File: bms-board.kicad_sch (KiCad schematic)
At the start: 1 part, among them U1 LTC6804-2

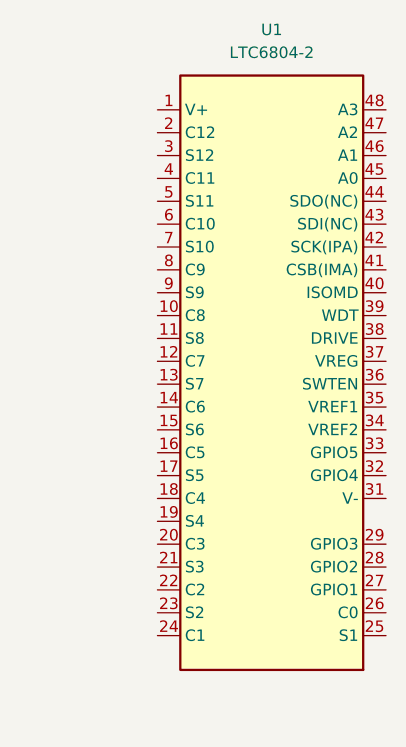
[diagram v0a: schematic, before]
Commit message: Release/0.1 (#8)
* feat: add 6804-2 kicad symbol

* feat: add 6804-2 kicad symbol (#3)

* TEMPLATE: add pull request description template

* feat: add automated git flow setup script

* update feature/add-cells branch to latest develop edition (#4)

* feat: add 6804-2 kicad symbol

* TEMPLATE: add pull request description template

* feat: add automated git flow setup script

* update feature/our-symbol-library branch to latest develop edition (#5)

* TEMPLATE: add pull request description template

* feat: add automated git flow setup script

* feat: a maybe working fixed wing schematic symbol library

* feat: add line to checkout dev branch when running setup script

* feat: fix FixedWing symbol library to include LTC6804-2

* refactor: verifying symbol library works, remove individual ltc6804-2 symbol

* feat: adding needed files

* feat: edit conflict in setup script

* Merging new develop into new feature (#6)

* feat: add 6804-2 kicad symbol

* TEMPLATE: add pull request description template

* feat: add automated git flow setup script

* update feature/our-symbol-library branch to latest develop edition (#5)

* TEMPLATE: add pull request description template

* feat: add automated git flow setup script

* feat: a maybe working fixed wing schematic symbol library

* feat: add line to checkout dev branch when running setup script

* feat: fix FixedWing symbol library to include LTC6804-2

* refactor: verifying symbol library works, remove individual ltc6804-2 symbol

* feat: adding needed files

* feat: edit conflict in setup script

---------

Co-authored-by: Ephram Cola Jacquin <89238547+ephram2004@users.noreply.github.com>
Co-authored-by: Ephram Cola Jacquin <ecolajacquin@gmail.com>

* fix: changed symbol for easier schematic design and orginization by pin logic

* docs: Update pull_request_template.md

---------

Co-authored-by: Ephram Cola Jacquin <89238547+ephram2004@users.noreply.gith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
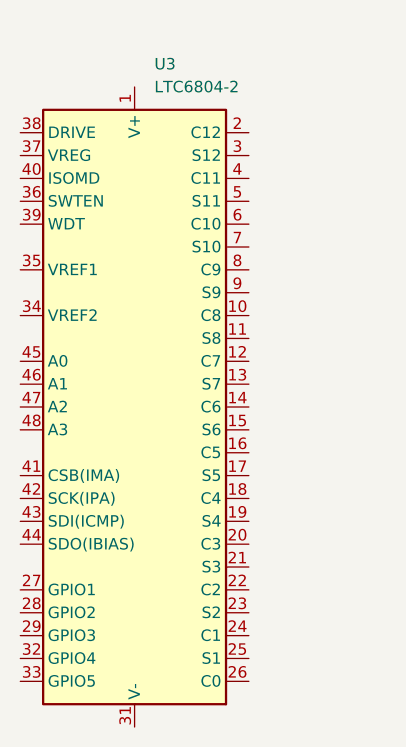
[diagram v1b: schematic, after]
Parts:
- removed U1: LTC6804-2, Package_SO:SSOP-48_5.3x12.8mm_P0.5mm, symbol Battery_Management:LTC6804-2
- added U3: LTC6804-2, Package_SO:SSOP-48_5.3x12.8mm_P0.5mm, symbol FixedWing:LTC6804-2
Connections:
- new net: U3.30 (V-), U3.31 (V-)
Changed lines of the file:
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@@
 (kicad_sch (version 20230121) (generator eeschema)
   (paper "A4")
-  (symbol (lib_id "Battery_Management:LTC6804-2") (at 148.59 92.71 0) (unit 1)
+  (symbol (lib_name "LTC6804-2_1") (lib_id "FixedWing:LTC6804-2") (at 133.35 96.52 0) (unit 1)
     (in_bom yes) (on_board yes) (dnp no) (fields_autoplaced)
-    (property "Reference" "U1" (at 148.59 54.61 0)
-      (effects (font (size 1.27 1.27)))
+    (property "Reference" "U3" (at 135.5441 58.42 0)
+      (effects (font (size 1.27 1.27)) (justify left))
     )
-    (property "Value" "LTC6804-2" (at 148.59 57.15 0)
-      (effects (font (size 1.27 1.27)))
+    (property "Value" "LTC6804-2" (at 135.5441 60.96 0)
+      (effects (font (size 1.27 1.27)) (justify left))
     )
-    (property "Footprint" "Package_SO:SSOP-48_5.3x12.8mm_P0.5mm" (at 148.59 130.81 0)
+    (property "Footprint" "Package_SO:SSOP-48_5.3x12.8mm_P0.5mm" (at 133.35 133.35 0)
       (effects (font (size 1.27 1.27)) hide)
     )
-    (property "Datasheet" "https://www.analog.com/media/en/technical-documentation/data-sheets/680412fc.pdf" (at 151.13 55.88 0)
+    (property "Datasheet" "https://www.analog.com/media/en/technical-documentation/data-sheets/680412fc.pdf" (at 147.32 62.23 0)
       (effects (font (size 1.27 1.27)) hide)
     )
+    (pin "37")
+    (pin "2")
+    (pin "39")
+    (pin "32")
+    (pin "36")
+    (pin "4")
+    (pin "41")
+    (pin "11")
+    (pin "20")
+    (pin "12")
+    (pin "21")
+    (pin "30")
+    (pin "33")
+    (pin "16")
     (pin "19")
-    (pin "20")
+    (pin "34")
+    (pin "40")
+    (pin "1")
+    (pin "13")
     (pin "17")
-    (pin "21")
-    (pin "39")
-    (pin "40")
-    (pin "16")
+    (pin "10")
+    (pin "18")
+    (pin "22")
+    (pin "26")
+    (pin "23")
+    (pin "24")
+    (pin "28")
     (pin "15")
-    (pin "22")
-    (pin "12")
-    (pin "44")
+    (pin "14")
+    (pin "27")
+    (pin "25")
+    (pin "29")
+    (pin "3")
+    (pin "35")
+    (pin "31")
+    (pin "38")
+    (pin "5")
+    (pin "42")
+    (pin "43")
+    (pin "48")
+    (pin "6")
+    (pin "7")
     (pin "45")
+    (pin "8")
+    (pin "9")
     (pin "46")
     (pin "47")
-    (pin "48")
-    (pin "23")
-    (pin "4")
-    (pin "11")
-    (pin "10")
-    (pin "5")
-    (pin "6")
-    (pin "7")
-    (pin "8")
-    (pin "9")
-    (pin "1")
-    (pin "24")
-    (pin "25")
-    (pin "26")
-    (pin "27")
-    (pin "28")
-    (pin "29")
-    (pin "3")
-    (pin "30")
-    (pin "31")
-    (pin "32")
-    (pin "33")
-    (pin "34")
-    (pin "35")
-    (pin "36")
-    (pin "37")
-    (pin "38")
-    (pin "13")
-    (pin "18")
-    (pin "2")
-    (pin "14")
-    (pin "41")
-    (pin "42")
-    (pin "43")
+    (pin "44")
     (instances
       (project "bms-board"
         (path "/8a7831d1-a913-4f04-8780-225d2234b41d"
-          (reference "U1") (unit 1)
+          (reference "U3") (unit 1)
         )
       )
